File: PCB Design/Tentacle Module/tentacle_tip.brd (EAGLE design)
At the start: 45.7 x 12.7 mm, 8 parts, among them U2 ADXL345PATRICK

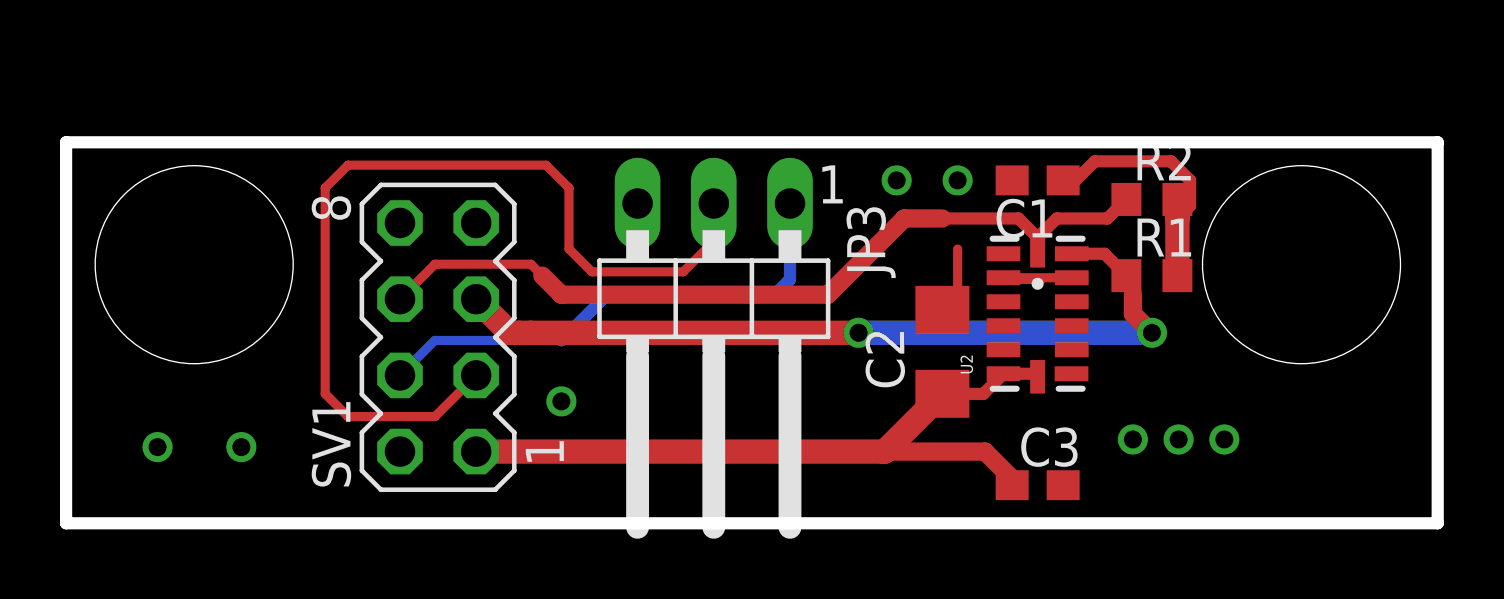
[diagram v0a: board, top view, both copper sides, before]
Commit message: Completed routing the tentacle tip board
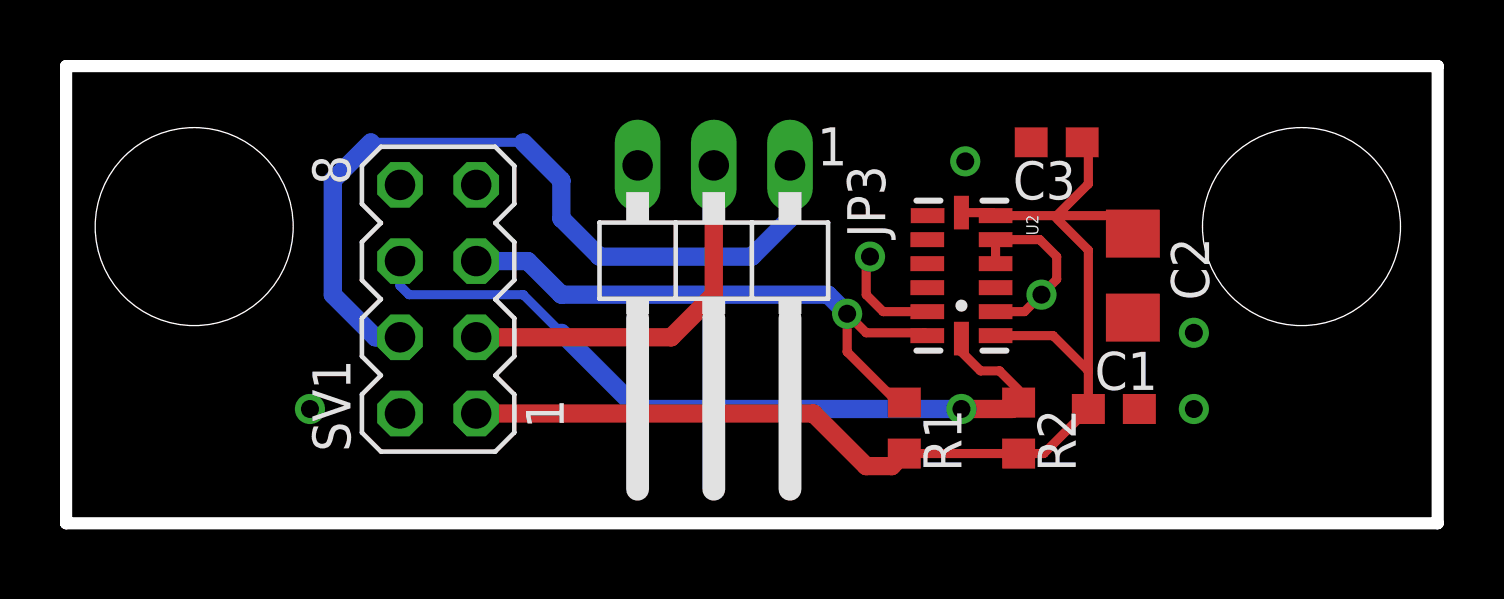
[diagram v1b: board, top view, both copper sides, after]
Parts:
- moved C3 11.4 mm to (33.0, 12.7), turned to 180 degrees
- moved R1 9.69 mm to (27.9, 3.17), turned to 270 degrees
- moved R2 8.82 mm to (31.8, 3.17), turned to 270 degrees
- moved C1 8.03 mm to (34.9, 3.81), turned to 0 degrees
- moved C2 6.84 mm to (35.6, 8.26), turned to 270 degrees
- moved U2 2.84 mm to (29.8, 8.26), turned to 270 degrees
- moved JP3 1.27 mm to (21.6, 8.12)
- moved SV1 1.27 mm to (12.4, 7.47)
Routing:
- net +5V: track 30.4 -> 12.8 mm
- net IR2: track 16.9 -> 27.0 mm
- net +3.3V: track 33.5 -> 41.3 mm
- net SDA: track 27.3 -> 19.9 mm, vias 2 -> 1
- net GND: track 5.80 -> 9.91 mm, vias 7 -> 6
- net SCL: track 27.4 -> 26.1 mm, vias 0 -> 1
- added copper zone on layer 1, net GND
- added copper zone on layer 16, net GND
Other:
- board size 45.7 x 12.7 mm -> 45.7 x 15.2 mm
